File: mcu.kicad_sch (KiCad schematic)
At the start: 14 parts

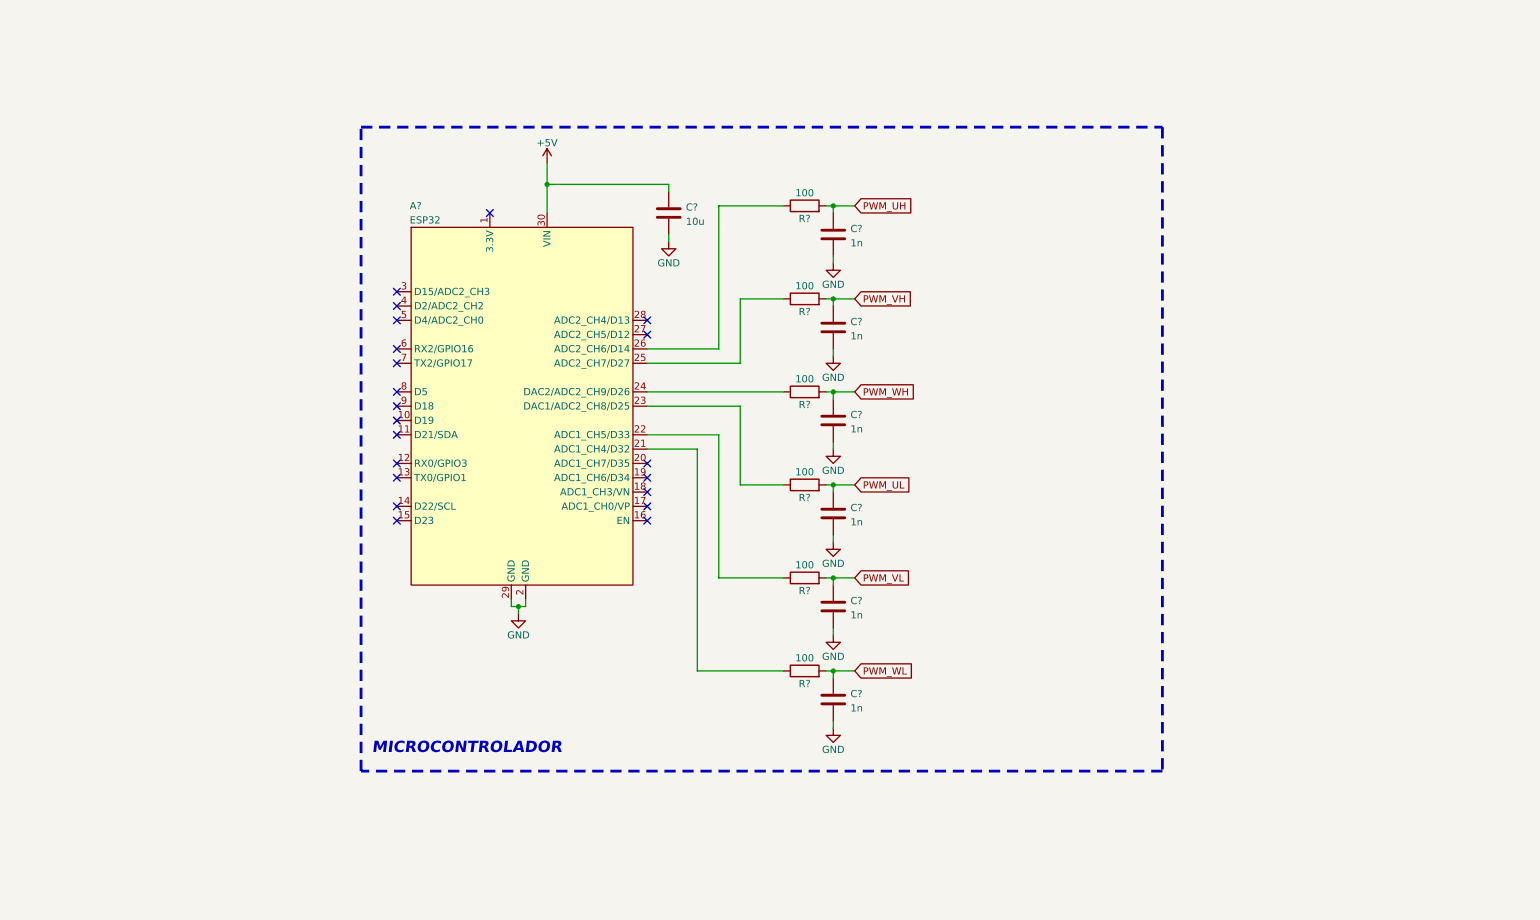
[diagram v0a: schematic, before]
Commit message: midsave
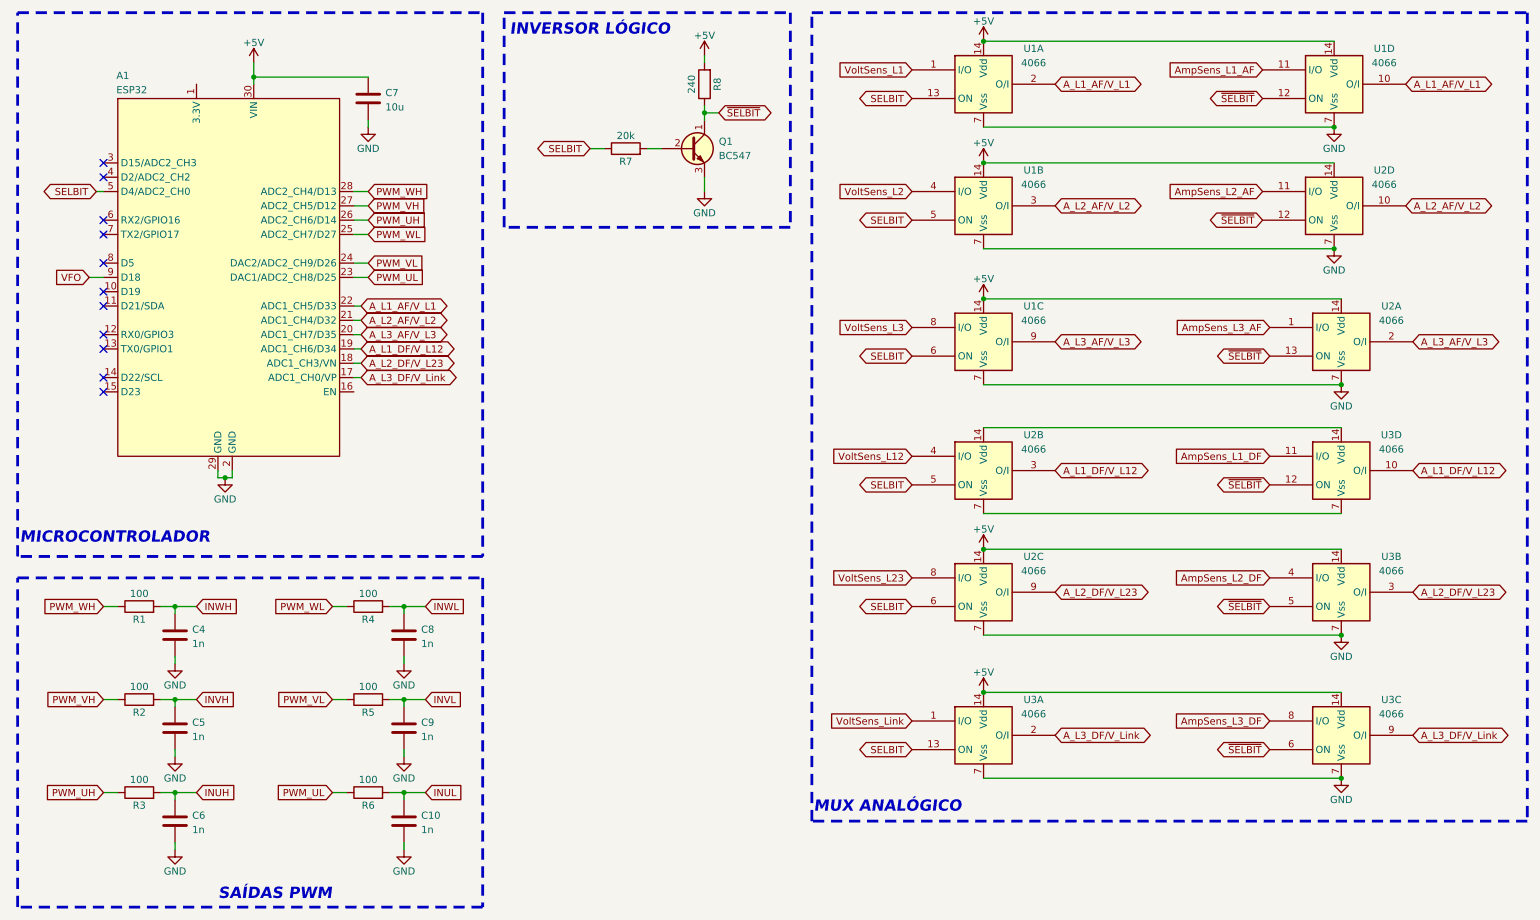
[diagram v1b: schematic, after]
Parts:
- removed A?: ESP32, PCM_SL_Development_Boards:DOIT_ESP32_DEVKIT_30Pins, symbol PCM_SL_Development_Board:ESP32_DevKit_V1_DOIT_30GPIOs
- removed C? (x6): 1n, symbol Device:C
- removed C?: 10u, symbol Device:C
- removed R? (x6): 100, symbol Device:R
- added A1: ESP32, PCM_SL_Development_Boards:DOIT_ESP32_DEVKIT_30Pins, symbol PCM_SL_Development_Board:ESP32_DevKit_V1_DOIT_30GPIOs
- added C10, C4, C5, C6, C8, C9: 1n, Capacitor_THT:C_Disc_D4.7mm_W2.5mm_P5.00mm, symbol Device:C
- added C7: 10u, Capacitor_THT:C_Radial_D6.3mm_H5.0mm_P2.50mm, symbol Device:C
- added Q1: BC547, PCM_Package_TO_SOT_THT_AKL:TO-92_HandSolder, symbol PCM_Transistor_BJT_AKL:BC547
- added R1, R2, R3, R4, R5, R6: 100, PCM_Resistor_THT_AKL:R_Axial_DIN0411_L9.9mm_D3.6mm_P20.32mm_Horizontal, symbol Device:R
- added R7: 20k, PCM_Resistor_THT_AKL:R_Axial_DIN0411_L9.9mm_D3.6mm_P20.32mm_Horizontal, symbol Device:R
- added R8: 240, PCM_Resistor_THT_AKL:R_Axial_DIN0411_L9.9mm_D3.6mm_P20.32mm_Horizontal, symbol Device:R
- added U1, U2, U3: 4066, Package_DIP:DIP-14_W7.62mm_LongPads, symbol 4xxx_IEEE:4066
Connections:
- net +5V: now also A1.30 (VIN), C7.1, R8.2, U1.14 (Vdd), U1.14 (Vdd), U1.14 (Vdd), U1.14 (Vdd), U2.14 (Vdd), U2.14 (Vdd), U2.14 (Vdd), U3.14 (Vdd), U3.14 (Vdd), U3.14 (Vdd)
- net GND: now also A1.2 (GND), A1.29 (GND), C10.2, C4.2, C5.2, C6.2, C7.2, C8.2, C9.2, Q1.3 (E), U1.7 (Vss), U1.7 (Vss), U1.7 (Vss), U1.7 (Vss), U2.7 (Vss), U2.7 (Vss), U2.7 (Vss), U3.7 (Vss), U3.7 (Vss), U3.7 (Vss)
- net PWM_UH: now also A1.26 (ADC2_CH6/D14), R3.1
- net PWM_UL: now also A1.23 (DAC1/ADC2_CH8/D25), R6.1
- net PWM_VH: now also A1.27 (ADC2_CH5/D12), R2.1
- net PWM_VL: now also A1.24 (DAC2/ADC2_CH9/D26), R5.1
- net PWM_WH: now also A1.28 (ADC2_CH4/D13), R1.1
- net PWM_WL: now also A1.25 (ADC2_CH7/D27), R4.1
- new net: Q1.2 (B), R7.2
- new net: U2.14 (Vdd), U3.14 (Vdd)
- new net: U2.7 (Vss), U3.7 (Vss)
- new net A_L1_AF/V_L1: A1.22 (ADC1_CH5/D33), U1.10 (O/I), U1.2 (O/I)
- new net A_L1_DF/V_L12: A1.19 (ADC1_CH6/D34), U2.3 (O/I), U3.10 (O/I)
- new net A_L2_AF/V_L2: A1.21 (ADC1_CH4/D32), U1.3 (O/I), U2.10 (O/I)
- new net A_L2_DF/V_L23: A1.18 (ADC1_CH3/VN), U2.9 (O/I), U3.3 (O/I)
- new net A_L3_AF/V_L3: A1.20 (ADC1_CH7/D35), U1.9 (O/I), U2.2 (O/I)
- new net A_L3_DF/V_Link: A1.17 (ADC1_CH0/VP), U3.2 (O/I), U3.9 (O/I)
- new net AmpSens_L1_AF: U1.11 (I/O)
- new net AmpSens_L1_DF: U3.11 (I/O)
- new net AmpSens_L2_AF: U2.11 (I/O)
- new net AmpSens_L2_DF: U3.4 (I/O)
- new net AmpSens_L3_AF: U2.1 (I/O)
- new net AmpSens_L3_DF: U3.8 (I/O)
- new net INUH: C6.1, R3.2
- new net INUL: C10.1, R6.2
- new net INVH: C5.1, R2.2
- new net INVL: C9.1, R5.2
- new net INWH: C4.1, R1.2
- new net INWL: C8.1, R4.2
- new net SELBIT: A1.5 (D4/ADC2_CH0), R7.1, U1.13 (ON), U1.5 (ON), U1.6 (ON), U2.5 (ON), U2.6 (ON), U3.13 (ON)
- new net VFO: A1.9 (D18)
- new net VoltSens_L1: U1.1 (I/O)
- new net VoltSens_L12: U2.4 (I/O)
- new net VoltSens_L2: U1.4 (I/O)
- new net VoltSens_L23: U2.8 (I/O)
- new net VoltSens_L3: U1.8 (I/O)
- new net VoltSens_Link: U3.1 (I/O)
- new net ~{SELBIT}: Q1.1 (C), R8.1, U1.12 (ON), U2.12 (ON), U2.13 (ON), U3.12 (ON), U3.5 (ON), U3.6 (ON)
- no-connect marks 21 -> 11
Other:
- note added: "INVERSOR LÓGICO"
- note added: "MUX ANALÓGICO"
- note added: "SAÍDAS PWM"
- company: (none) -> Autor: José Fonseca
- title: (none) -> Microcontrolador
